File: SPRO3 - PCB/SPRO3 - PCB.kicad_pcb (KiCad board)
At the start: 2 copper layers, 100 x 80 mm, 42 parts, among them J1 Power Input, J10 Conn_01x03_Pin, J11 Conn_01x03_Pin, J12 Conn_01x03_Pin, J13 Conn_01x03_Pin, J14 Conn_01x03_Pin, J15 Conn_01x03_Pin, J2 2nd PCB, J3 Servo Motor, J4 L298N Module, J5 Gate Sensor, J6 Magnometer, J7 GPS Module, J8 Conn_01x03_Pin, J9 Conn_01x03_Pin, SW1 SW_SPDT, U2 CD4051B

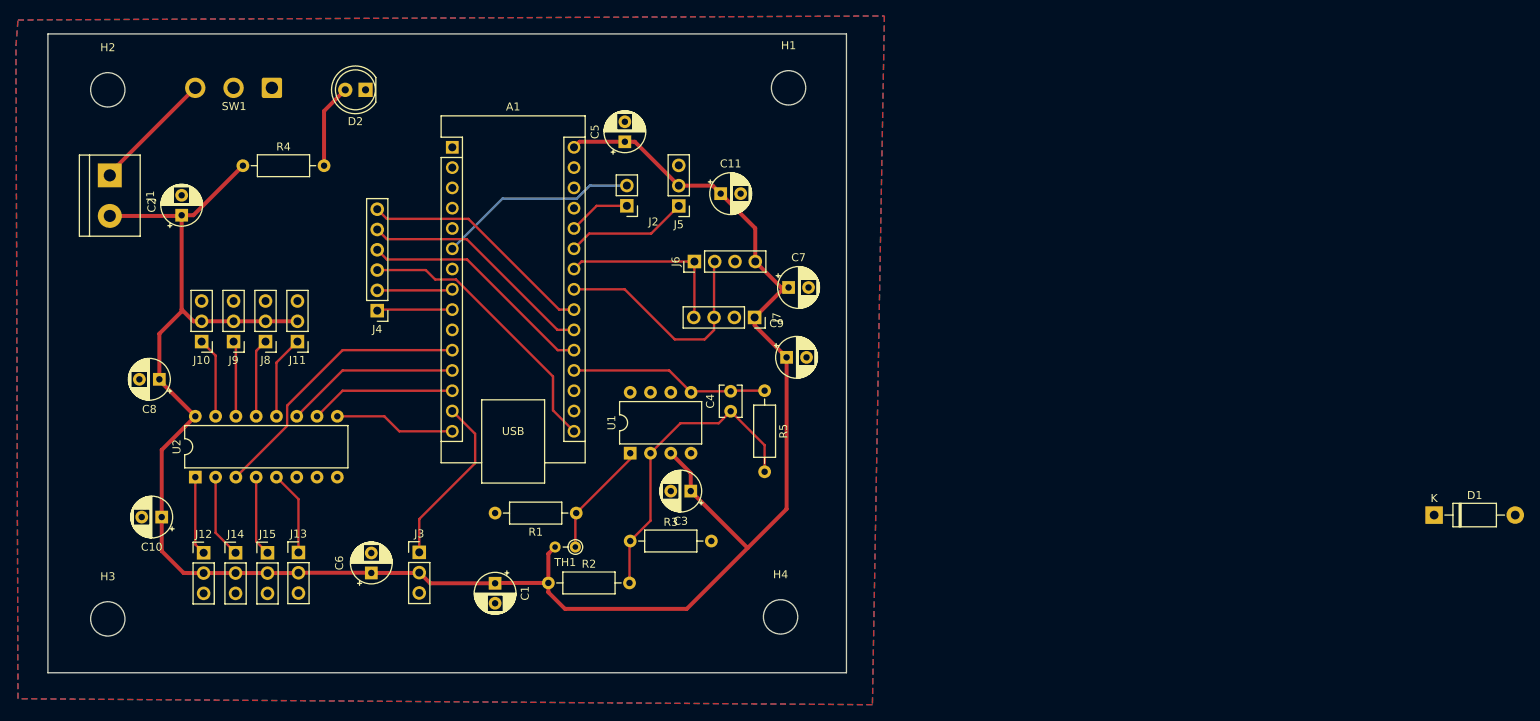
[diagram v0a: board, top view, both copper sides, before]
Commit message: finished the PCB board designs
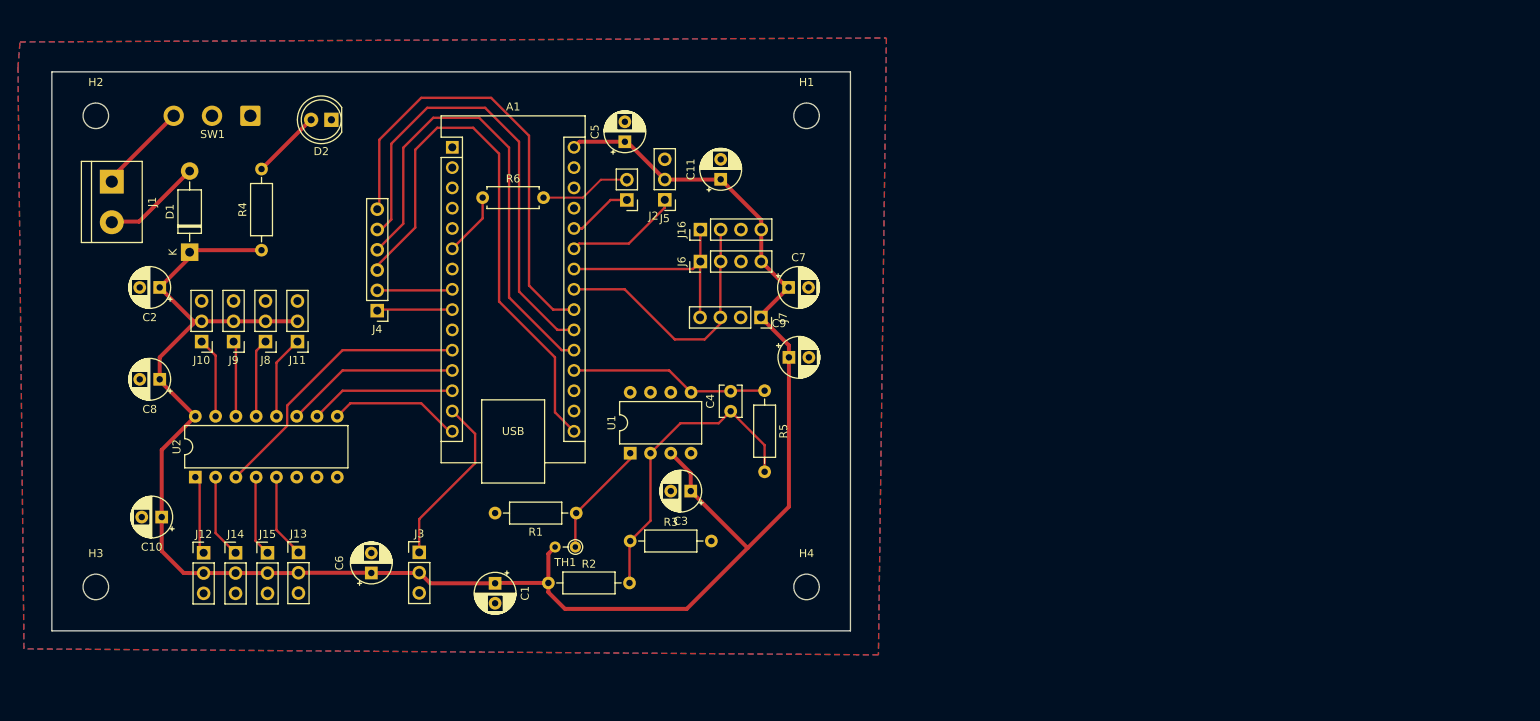
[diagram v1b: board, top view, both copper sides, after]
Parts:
- added J16: Spare I2C PINS, Connector_PinHeader_2.54mm:PinHeader_1x04_P2.54mm_Vertical, F.Cu at (152.0, 94.5)
- added R6: 20, Resistor_THT:R_Axial_DIN0207_L6.3mm_D2.5mm_P7.62mm_Horizontal, F.Cu at (124.7, 90.5)
- H1, H2, H3, H4: footprint MountingHole:MountingHole_4.3mm_M4 -> MountingHole:MountingHole_3.2mm_M3
- moved D1 159.3 mm to (88.0, 97.3), turned to 90 degrees
- moved R4 10.8 mm to (97.0, 97.1), turned to 90 degrees
- moved C2 9.45 mm to (84.2, 101.8), turned to 180 degrees
- moved D2 5.69 mm to (105.8, 80.8)
- moved H4 4.96 mm to (165.2, 139.2)
- moved SW1 4.42 mm to (95.6, 80.2)
- moved H3 4.27 mm to (76.2, 139.2)
- moved H1 4.16 mm to (165.2, 80.2)
- moved H2 3.58 mm to (76.2, 80.2)
- moved J5 1.91 mm to (147.5, 90.8)
- moved C11 1.79 mm to (154.5, 88.2), turned to 90 degrees
- moved J1 0.83 mm to (78.2, 88.5)
- moved J7 0.79 mm to (159.5, 105.5)
- moved J6 0.75 mm to (152.0, 98.5)
- moved J2 0.73 mm to (142.8, 90.8)
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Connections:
- D1 pad 1: unconnected-(D1-K-Pad1) -> +5V
- D1 pad 2: unconnected-(D1-A-Pad2) -> Net-(D1-A)
- J1 pad 2: +5V -> Net-(D1-A)
- J2 pad 2: /OC2B -> Net-(J2-Pin_2)
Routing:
- net /IN1: track 35.5 -> 68.7 mm
- net /IN3: track 29.8 -> 60.1 mm
- net /IN4: track 29.8 -> 59.0 mm
- net /IN2: track 29.8 -> 57.3 mm
- net /OC2B: track 25.1 -> 7.97 mm
- net +5V: track 257.8 -> 245.2 mm
- net Net-(D1-A): track 0.00 -> 12.4 mm
- net Net-(J2-Pin_2): track 0.00 -> 11.7 mm
- net /SCL: track 22.5 -> 27.3 mm
- net /SDA: track 29.2 -> 33.7 mm
- net Net-(J1-Pin_1): track 15.4 -> 11.5 mm
- net Net-(D2-A): track 10.6 -> 8.77 mm
- net /C: track 15.2 -> 16.5 mm
- net /ADC6: track 15.3 -> 14.5 mm
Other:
- board size 100 x 80 mm -> 100 x 70 mm
